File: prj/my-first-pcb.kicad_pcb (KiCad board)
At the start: 4 copper layers, 31 x 50 mm, 50 parts, among them J1 Conn_01x16_Pin, J2 Conn_01x16_Pin, J3 USB_C_Receptacle_PowerOnly_6P, J4 TagConnect, SW1 TSA063G60-250, SW2 TSA063G60-250, U1 AP61302Z6, U2 nRF52832-QFxx, Y1 32.768kHz, Y2 32MHz

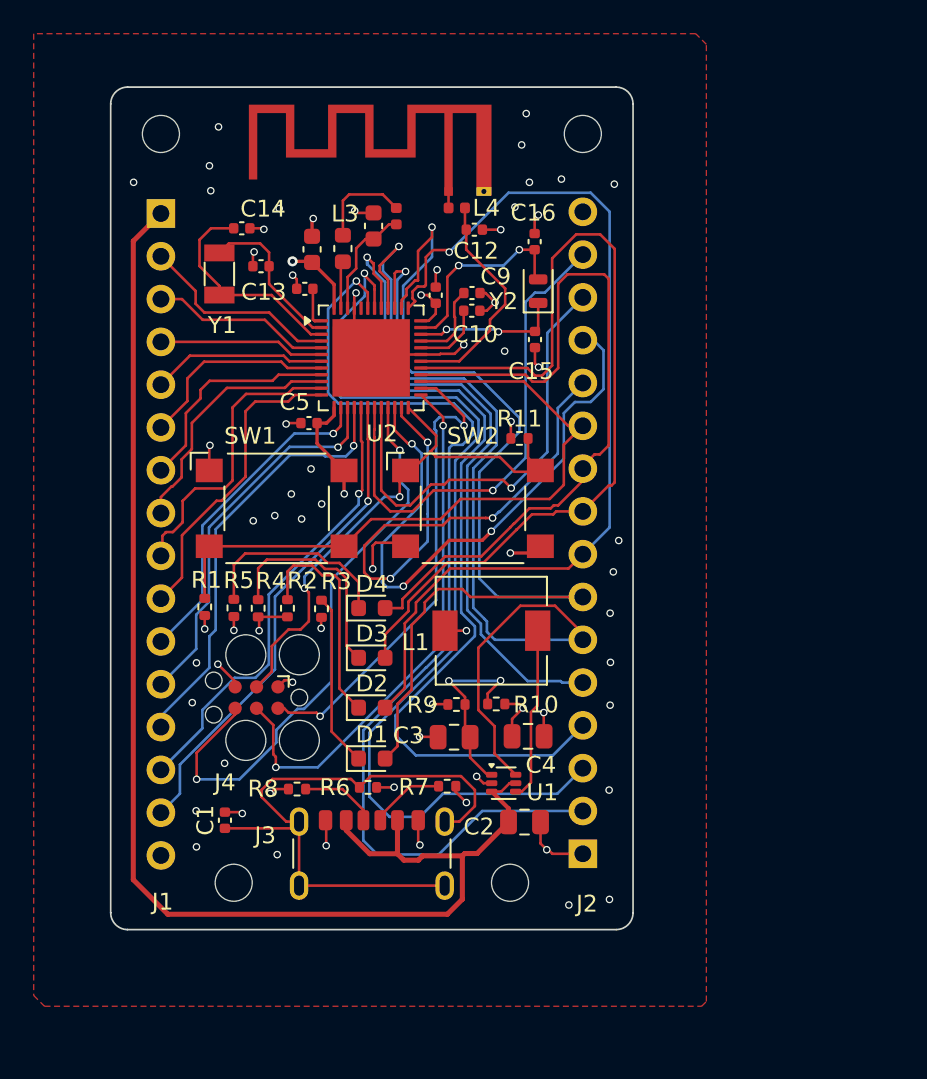
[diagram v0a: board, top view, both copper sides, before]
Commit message: PCB routed trial 2
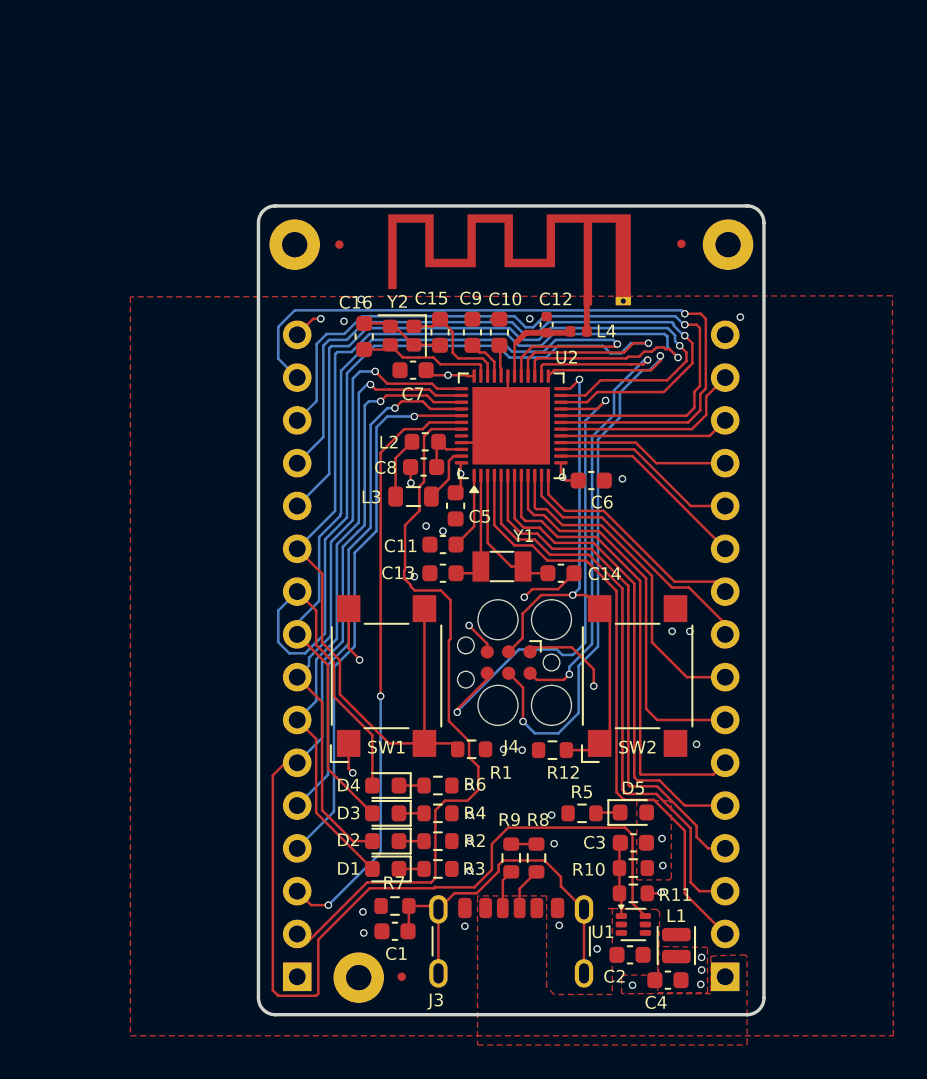
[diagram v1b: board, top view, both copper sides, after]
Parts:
- removed the REF** at (137.0, 119.6)
- removed the REF** at (141.3, 75.2)
- removed the REF** at (120.6, 119.6)
- removed the REF** at (116.3, 75.2)
- added ?: , , F.Cu at (149.9, 81.7)
- added ?: , , F.Cu at (124.2, 81.7)
- added ?: , , F.Cu at (128.0, 125.2)
- added ?: , , F.Cu at (126.8, 81.7)
- added ?: , , F.Cu at (147.1, 81.7)
- added D5: LED RED, LED_SMD:LED_0603_1608Metric, F.Cu at (144.3, 115.4)
- added R12: 10k, Resistor_SMD:R_0603_1608Metric, F.Cu at (139.5, 111.7)
- added REF**: Fiducial_0.5mm_Mask1.5mm, Fiducial:Fiducial_0.5mm_Mask1.5mm, F.Cu at (130.5, 125.2)
- AE1: value Antenna -> Antenna_Shield
- C1, C10, C11, C5, C6, C9: footprint Capacitor_SMD:C_0402_1005Metric -> Capacitor_SMD:C_0603_1608Metric
- C13, C14: value 12p -> 18p; footprint Capacitor_SMD:C_0402_1005Metric -> Capacitor_SMD:C_0603_1608Metric
- C15, C16: value 12p -> 10p; footprint Capacitor_SMD:C_0402_1005Metric -> Capacitor_SMD:C_0603_1608Metric
- C2, C4: footprint Capacitor_SMD:C_0805_2012Metric -> Capacitor_SMD:C_0603_1608Metric
- C3: value 33uF -> 33pF; footprint Capacitor_SMD:C_0805_2012Metric -> Capacitor_SMD:C_0603_1608Metric
- D1: value LED -> LED RED
- D2: value LED -> LED BLUE
- D3: value LED -> LED YELLOW
- D4: value LED -> LED GREEN
- L1: footprint Inductor_SMD:L_6.3x6.3_H3 -> Inductor_SMD:L_Changjiang_FTC201610S
- L2: footprint Inductor_SMD:L_0402_1005Metric -> Inductor_SMD:L_0603_1608Metric
- L3: footprint Inductor_SMD:L_0603_1608Metric -> Inductor_SMD:L_0805_2012Metric
- R1: value 470 -> 10k; footprint Resistor_SMD:R_0402_1005Metric -> Resistor_SMD:R_0603_1608Metric
- R10: value 44k2 -> 200k; footprint Resistor_SMD:R_0402_1005Metric -> Resistor_SMD:R_0603_1608Metric
- R11: value 10k -> 44k2; footprint Resistor_SMD:R_0402_1005Metric -> Resistor_SMD:R_0603_1608Metric
- R2, R3, R4, R8: footprint Resistor_SMD:R_0402_1005Metric -> Resistor_SMD:R_0603_1608Metric
- R5: value 1k -> 10k; footprint Resistor_SMD:R_0402_1005Metric -> Resistor_SMD:R_0603_1608Metric
- R6: value 1M -> 1k; footprint Resistor_SMD:R_0402_1005Metric -> Resistor_SMD:R_0603_1608Metric
- R7: value 5k1 -> 1M; footprint Resistor_SMD:R_0402_1005Metric -> Resistor_SMD:R_0603_1608Metric
- R9: value 200k -> 5k1; footprint Resistor_SMD:R_0402_1005Metric -> Resistor_SMD:R_0603_1608Metric
- Y1: value 32.768kHz -> Q13FC13500004
- Y2: value 32MHz -> XL7EL89CKI-111YLC-32M; footprint Crystal:Crystal_SMD_2012-2Pin_2.0x1.2mm -> Crystal:Crystal_SMD_2016-4Pin_2.0x1.6mm
- moved J1 42.6 mm to (149.7, 125.2), turned to 0 degrees
- moved J2 31.3 mm to (124.3, 125.2)
- moved C14 27.9 mm to (140.0, 101.2)
- moved R11 27.8 mm to (144.3, 120.2)
- moved Y1 24.1 mm to (136.5, 100.8), turned to 180 degrees
- moved R5 24.0 mm to (141.2, 115.5), turned to 180 degrees
- moved L1 21.7 mm to (146.8, 123.3), turned to -90 degrees
- moved C13 21.2 mm to (133.0, 101.2)
- moved R1 18.0 mm to (134.7, 111.7), turned to 0 degrees
- moved C11 17.3 mm to (133.0, 99.5)
- moved R3 16.9 mm to (132.7, 118.8), turned to 0 degrees
- moved C4 16.7 mm to (146.3, 125.4)
- moved R2 16.5 mm to (132.7, 117.1), turned to 0 degrees
- moved R4 16.2 mm to (132.7, 115.5), turned to 0 degrees
- moved L3 15.3 mm to (131.2, 96.7), turned to 0 degrees
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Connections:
- net Net-(AE1-A) renamed /MCU/RF
- AE1 pad 2: (no net) -> GND
- R10 pad 1: Net-(U1-FB) -> +3V3
- R10 pad 2: GND -> Net-(U1-FB)
- R11 pad 1: +3V3 -> Net-(U1-FB)
- R11 pad 2: /MCU/NRST -> GND
- R5 pad 1: Net-(D4-K) -> Net-(D5-K)
- R6 pad 1: Net-(J3-SHIELD) -> Net-(D4-K)
- R7 pad 1: Net-(J3-CC2) -> Net-(J3-SHIELD)
- R8 pad 1: GND -> Net-(J3-CC2)
- R8 pad 2: Net-(J3-CC1) -> GND
- R9 pad 1: +3V3 -> GND
- R9 pad 2: Net-(U1-FB) -> Net-(J3-CC1)
- Y2 pad 2: /MCU/XC2 -> GND
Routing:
- net +5V: track 81.3 -> 1.03 mm
- net GND: track 50.9 -> 20.4 mm, vias 61 -> 28
- net /MCU/MCU_IO18: track 40.4 -> 70.9 mm, vias 0 -> 1
- net /MCU/MCU_IO23: track 52.6 -> 77.3 mm
- net /MCU/MCU_IO0: track 12.1 -> 35.9 mm
- net /MCU/MCU_IO1: track 10.7 -> 34.1 mm
- net /MCU/MCU_IO26: track 58.8 -> 35.9 mm, vias 1 -> 2
- net /MCU/MCU_IO22: track 60.0 -> 38.2 mm
- net /MCU/MCU_IO2: track 9.84 -> 30.9 mm
- net /MCU/MCU_IO25: track 52.7 -> 32.3 mm
- net /MCU/MCU_IO19: track 45.0 -> 64.5 mm, vias 0 -> 1
- net /MCU/MCU_IO3: track 10.4 -> 28.8 mm
- net /MCU/MCU_IO21: track 56.0 -> 38.4 mm
- net /MCU/MCU_IO13: track 29.1 -> 11.7 mm, vias 1 -> 0
- net /MCU/MCU_IO27: track 60.9 -> 43.7 mm, vias 1 -> 0
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- added copper zone on F.Cu, net +3V3
- added copper zone on F.Cu, net +5V
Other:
- board size 31 x 50 mm -> 30 x 48 mm
